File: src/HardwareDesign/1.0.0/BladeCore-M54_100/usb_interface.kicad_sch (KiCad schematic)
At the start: 22 parts, among them IC7 TPS74801DRCT, IC8 SN74LVC1G97QDCKRQ1

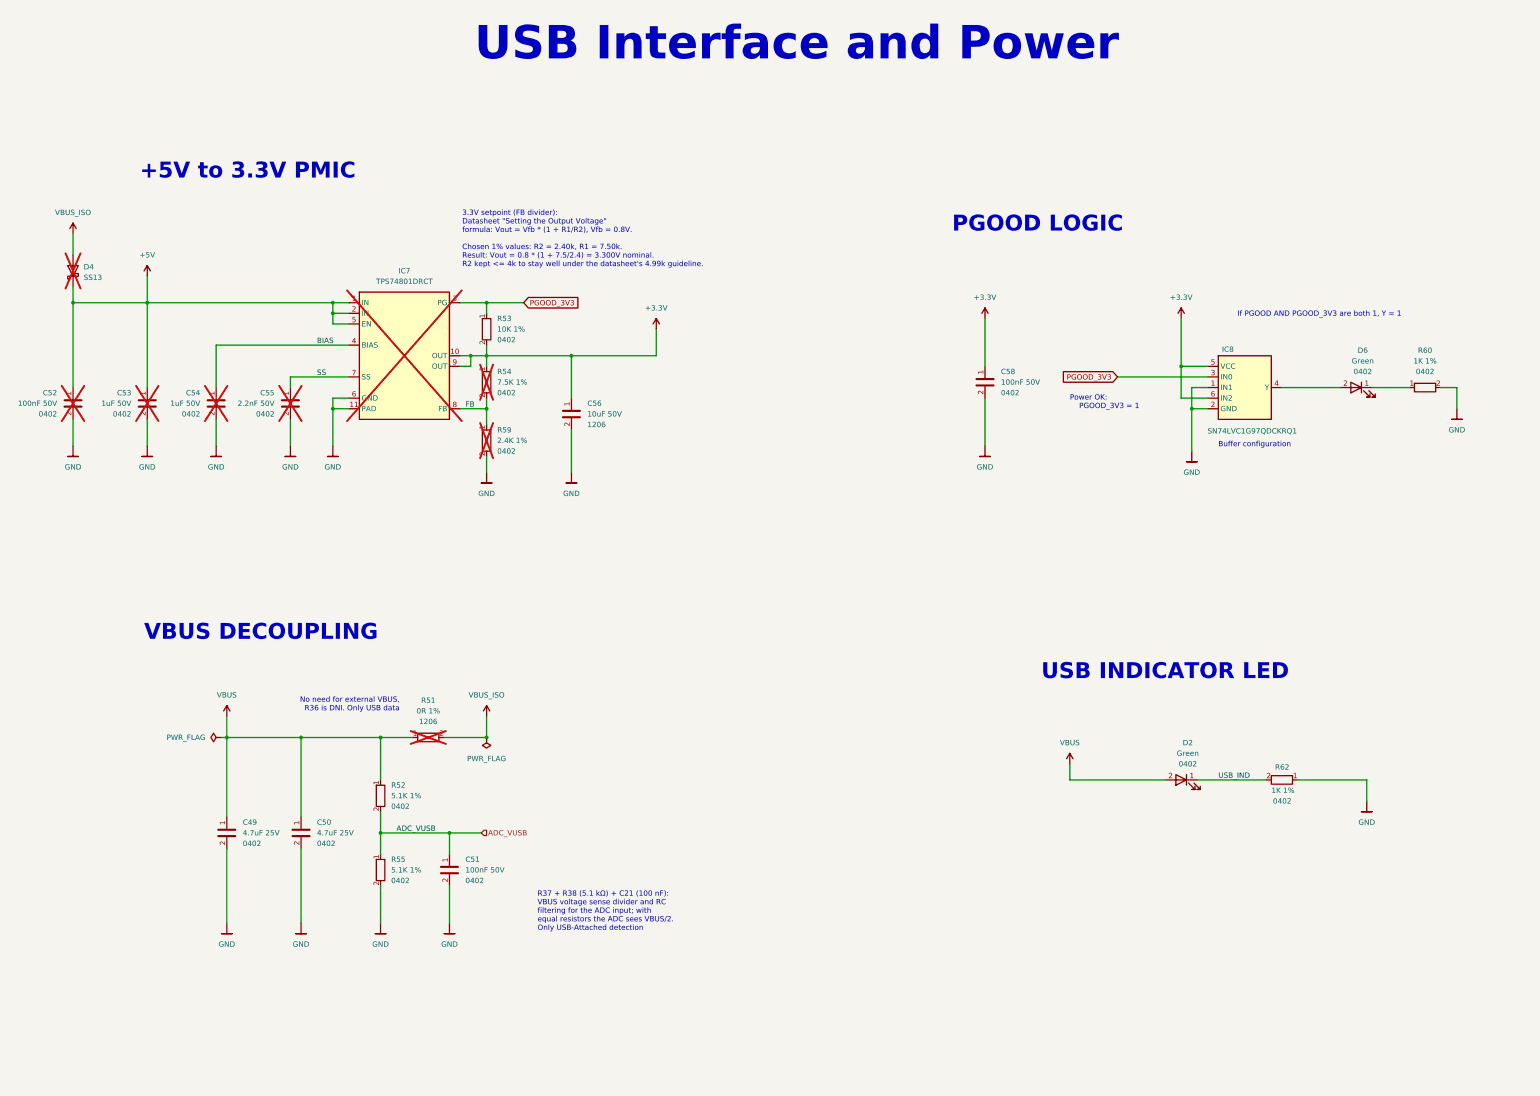
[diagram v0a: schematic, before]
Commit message: M54 rework
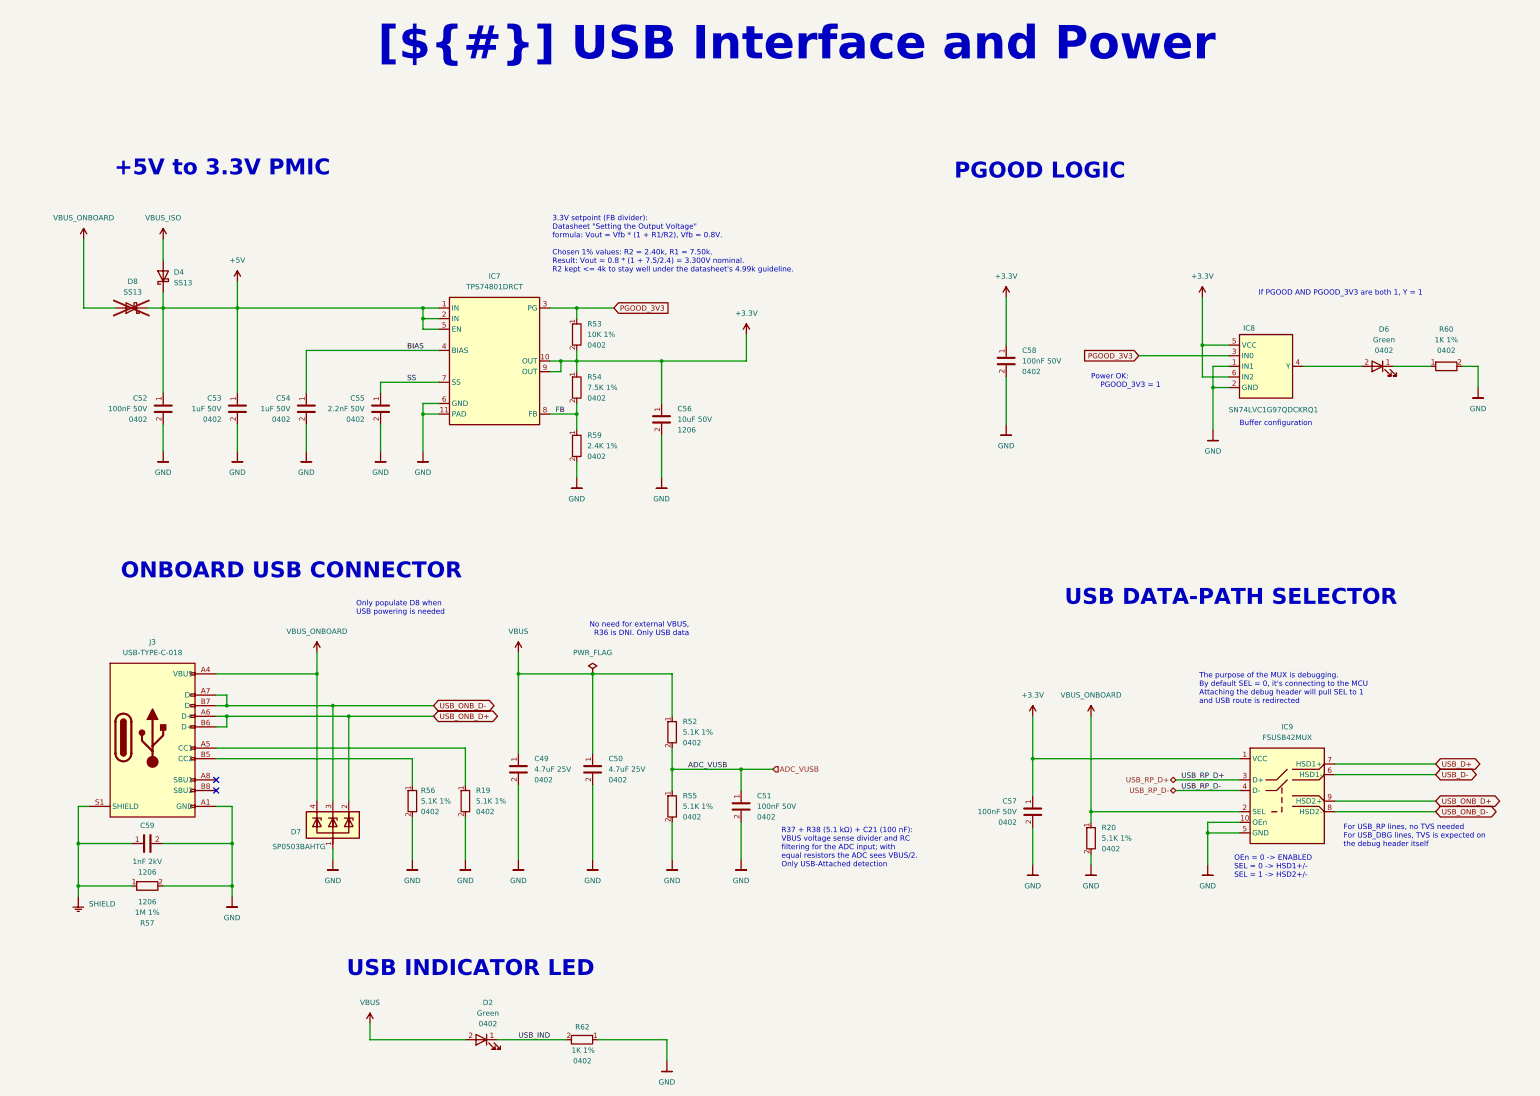
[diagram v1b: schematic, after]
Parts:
- removed R51: 0R 1%, Resistor_SMD:R_1206_3216Metric, symbol DS_Resistor_1206:0R 1% 1206
- added C57: 100nF 50V, Capacitor_SMD:C_0402_1005Metric, symbol DS_Capacitor_0402:100nF 50V 0402
- added C59: 1nF 2kV, Capacitor_SMD:C_1206_3216Metric, symbol DS_Capacitor_1206:1nF 2kV 1206
- added D7: SP0503BAHTG, DS_Diode:SOT143, symbol DS_Diode:SP0503BAHTG
- added D8: SS13, Diode_SMD:D_SMA, symbol Diode:SS13
- added IC9: FSUSB42MUX, DS_Peripherals:MSOP-10_3x3mm_P0.5mm, symbol DS_Peripherals:FSUSB42MUX
- added J3: USB-TYPE-C-018, DS_Connector:USB_C_Receptacle_HCTL_HC-TYPE-C-16P-01A, symbol DS_Connector:USB-C
- added R19, R20, R56: 5.1K 1%, Resistor_SMD:R_0402_1005Metric, symbol DS_Resistor_0402:5.1K 1% 0402
- added R57: 1M 1%, Resistor_SMD:R_1206_3216Metric, symbol DS_Resistor_1206:1M 1% 1206
- C52, C53, C54, C55, D4, IC7, R54, R59: now fitted; now in the parts list
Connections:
- net +3.3V: now also C57.1, IC9.1 (VCC)
- net +5V: now also D8.1 (K)
- net GND: now also C57.2, C59.2, D7.1, IC9.10 (OEn), IC9.5 (GND), J3.A1 (GND), J3.A12 (GND), J3.B1 (GND), J3.B12 (GND), R19.2, R20.2, R56.2, R57.2
- new net: J3.A5 (CC1), R19.1
- new net: J3.B5 (CC2), R56.1
- new net SHIELD: C59.1, J3.S1 (SHIELD), R57.1
- new net USB_D+: IC9.7 (HSD1+)
- new net USB_D-: IC9.6 (HSD1-)
- new net USB_ONB_D+: D7.2, IC9.9 (HSD2+), J3.A6 (D+), J3.B6 (D+)
- new net USB_ONB_D-: D7.3, IC9.8 (HSD2-), J3.A7 (D-), J3.B7 (D-)
- new net USB_RP_D+: IC9.3 (D+)
- new net USB_RP_D-: IC9.4 (D-)
- new net VBUS_ONBOARD: D7.4, D8.2 (A), IC9.2 (SEL), J3.A4 (VBUS), J3.A9 (VBUS), J3.B4 (VBUS), J3.B9 (VBUS), R20.1
- no-connect marks 0 -> 2
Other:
- note added: "For USB_RP lines, no TVS needed For USB_DBG lines, TVS is expected on the debug header itself"
- note added: "OEn = 0 -> ENABLED SEL = 0 -> HSD1+/- SEL = 1 -> HSD2+/-"
- note added: "ONBOARD USB CONNECTOR"
- note added: "Only populate D8 when USB powering is needed"
- note added: "The purpose of the MUX is debugging. By default SEL = 0, it's connecting to the MCU Attaching the debug header will pull SEL to 1 and USB route is redirected"
- note added: "USB DATA-PATH SELECTOR"
- note removed: "VBUS DECOUPLING"
- company: DvidMakesThings -> ${COMPANY}
- moved on the sheet: C49, C50, C51, C56, C58, D2, D6, IC8, R52, R53, R55, R60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
